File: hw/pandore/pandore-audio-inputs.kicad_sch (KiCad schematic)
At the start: 2 parts, among them J4 XLR+TRS6.35+3SW, J5 XLR+TRS6.35+3SW

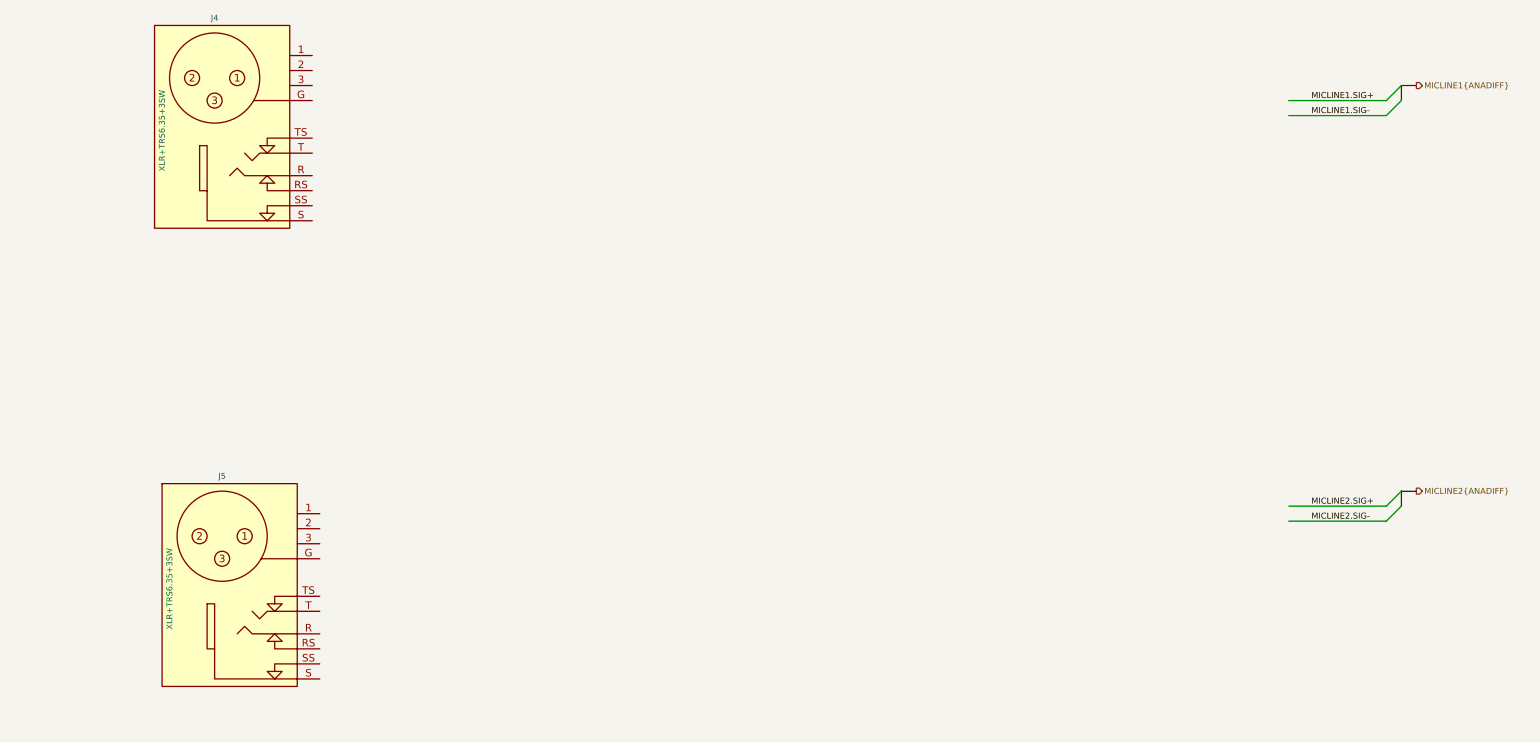
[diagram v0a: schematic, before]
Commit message: lots of work done all around
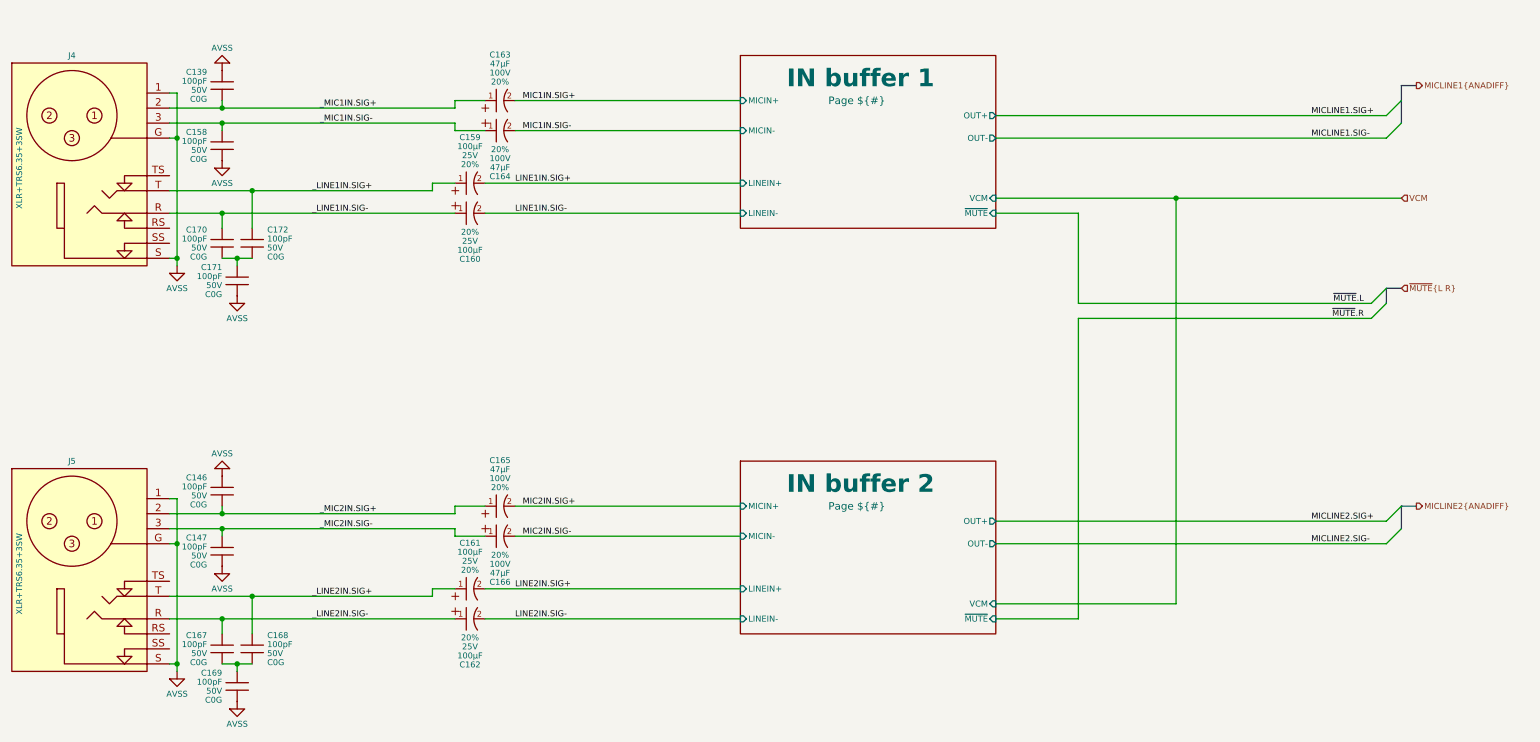
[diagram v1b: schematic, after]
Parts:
- added C139, C146, C147, C158, C167, C168, C169, C170, C171, C172: ${Capacitance}, ${Voltage}, ${Dielectric}, reekilib_cap:CAPC1608, symbol reekilib_cap:cap
- added C159, C160, C161, C162, C163, C164, C165, C166: ${Capacitance}, ${Voltage}, ${Tolerance}, reekilib_cap:CAPAE630Xxxx, symbol reekilib_cap:cap_pol
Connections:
- net AVSS: now reaches J4.1
- net AVSS: now also J4.G, J4.S, J5.1, J5.G, J5.S, C139.2, C146.2, C147.1, C158.1, C169.1, C171.1
- net _MIC1IN.SIG+: now reaches J4.2
- net _MIC1IN.SIG+: now also C139.1, C163.1 (+)
- net _MIC1IN.SIG-: now reaches J4.3
- net _MIC1IN.SIG-: now also C158.2, C164.1 (+)
- net _LINE1IN.SIG-: now reaches J4.R
- net _LINE1IN.SIG-: now also C160.1 (+), C170.2
- net _LINE1IN.SIG+: now reaches J4.T
- net _LINE1IN.SIG+: now also C159.1 (+), C172.2
- net _MIC2IN.SIG+: now reaches J5.2
- net _MIC2IN.SIG+: now also C146.1, C165.1 (+)
- net _MIC2IN.SIG-: now reaches J5.3
- net _MIC2IN.SIG-: now also C147.2, C166.1 (+)
- net _LINE2IN.SIG-: now reaches J5.R
- net _LINE2IN.SIG-: now also C162.1 (+), C167.2
- net _LINE2IN.SIG+: now reaches J5.T
- net _LINE2IN.SIG+: now also C161.1 (+), C168.2
- new net: C167.1, C168.1, C169.2
- new net: C170.1, C171.2, C172.1
- new net LINE1IN.SIG+: C159.2 (-)
- new net LINE1IN.SIG-: C160.2 (-)
- new net LINE2IN.SIG+: C161.2 (-)
- new net LINE2IN.SIG-: C162.2 (-)
- new net MIC1IN.SIG+: C163.2 (-)
- new net MIC1IN.SIG-: C164.2 (-)
- new net MIC2IN.SIG+: C165.2 (-)
- new net MIC2IN.SIG-: C166.2 (-)
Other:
- added sheet IN buffer 1 (pandore-audio-inbuf.kicad_sch)
- added sheet IN buffer 2 (pandore-audio-inbuf.kicad_sch)
- moved on the sheet: J4, J5
